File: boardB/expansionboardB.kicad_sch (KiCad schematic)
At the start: 45 parts, among them J1 USB_C_Receptacle, J3 HDMI_A, SW4 ESPPROG, U1 ESP32-S3-WROOM-1, U2 GPIO_U2, U4 GPIO_U4, U5 SII1136CTU, U7 MAX20022ATIA+T, t1V2 1V2_TEST, t3V3 3V3_TEST

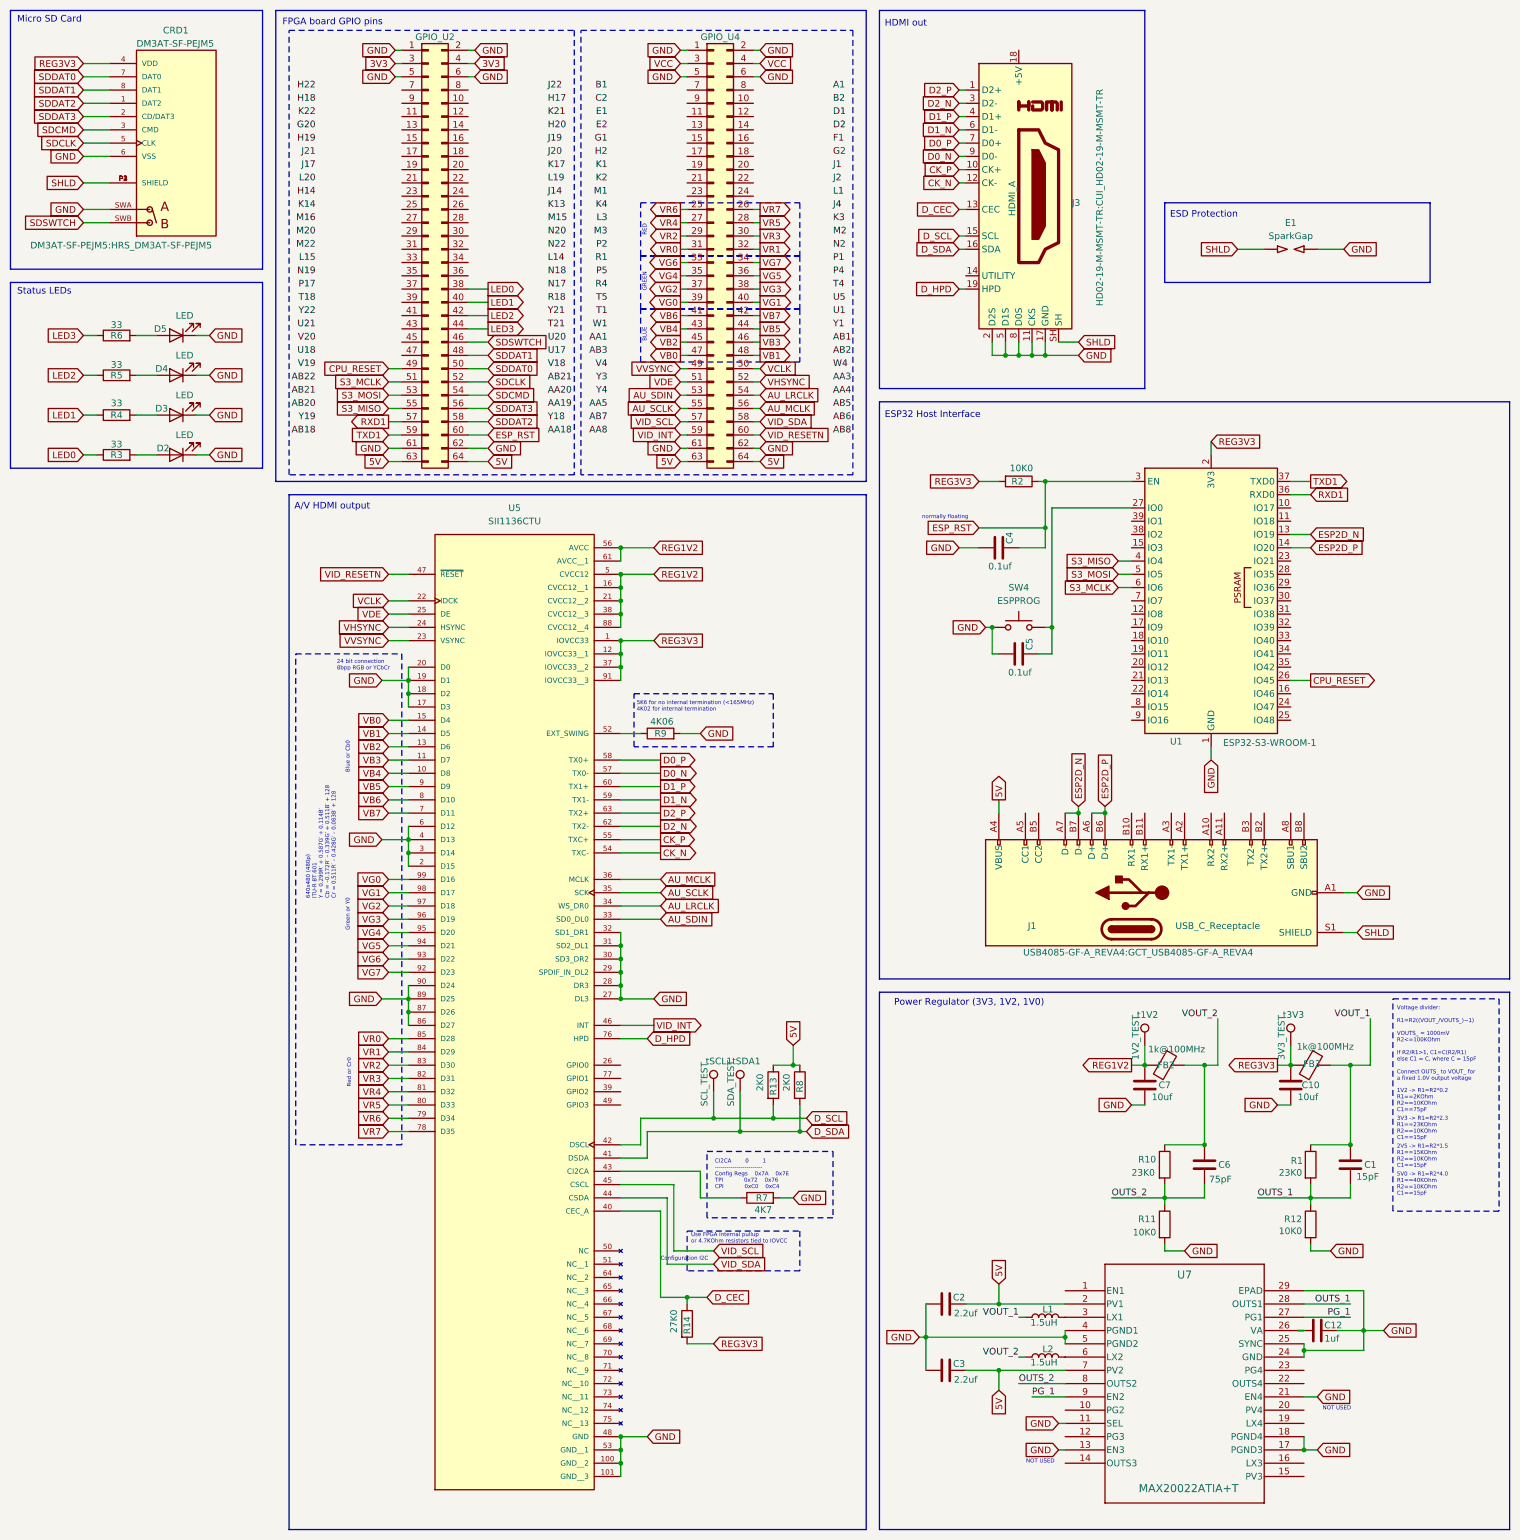
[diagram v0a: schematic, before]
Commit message: New board updates
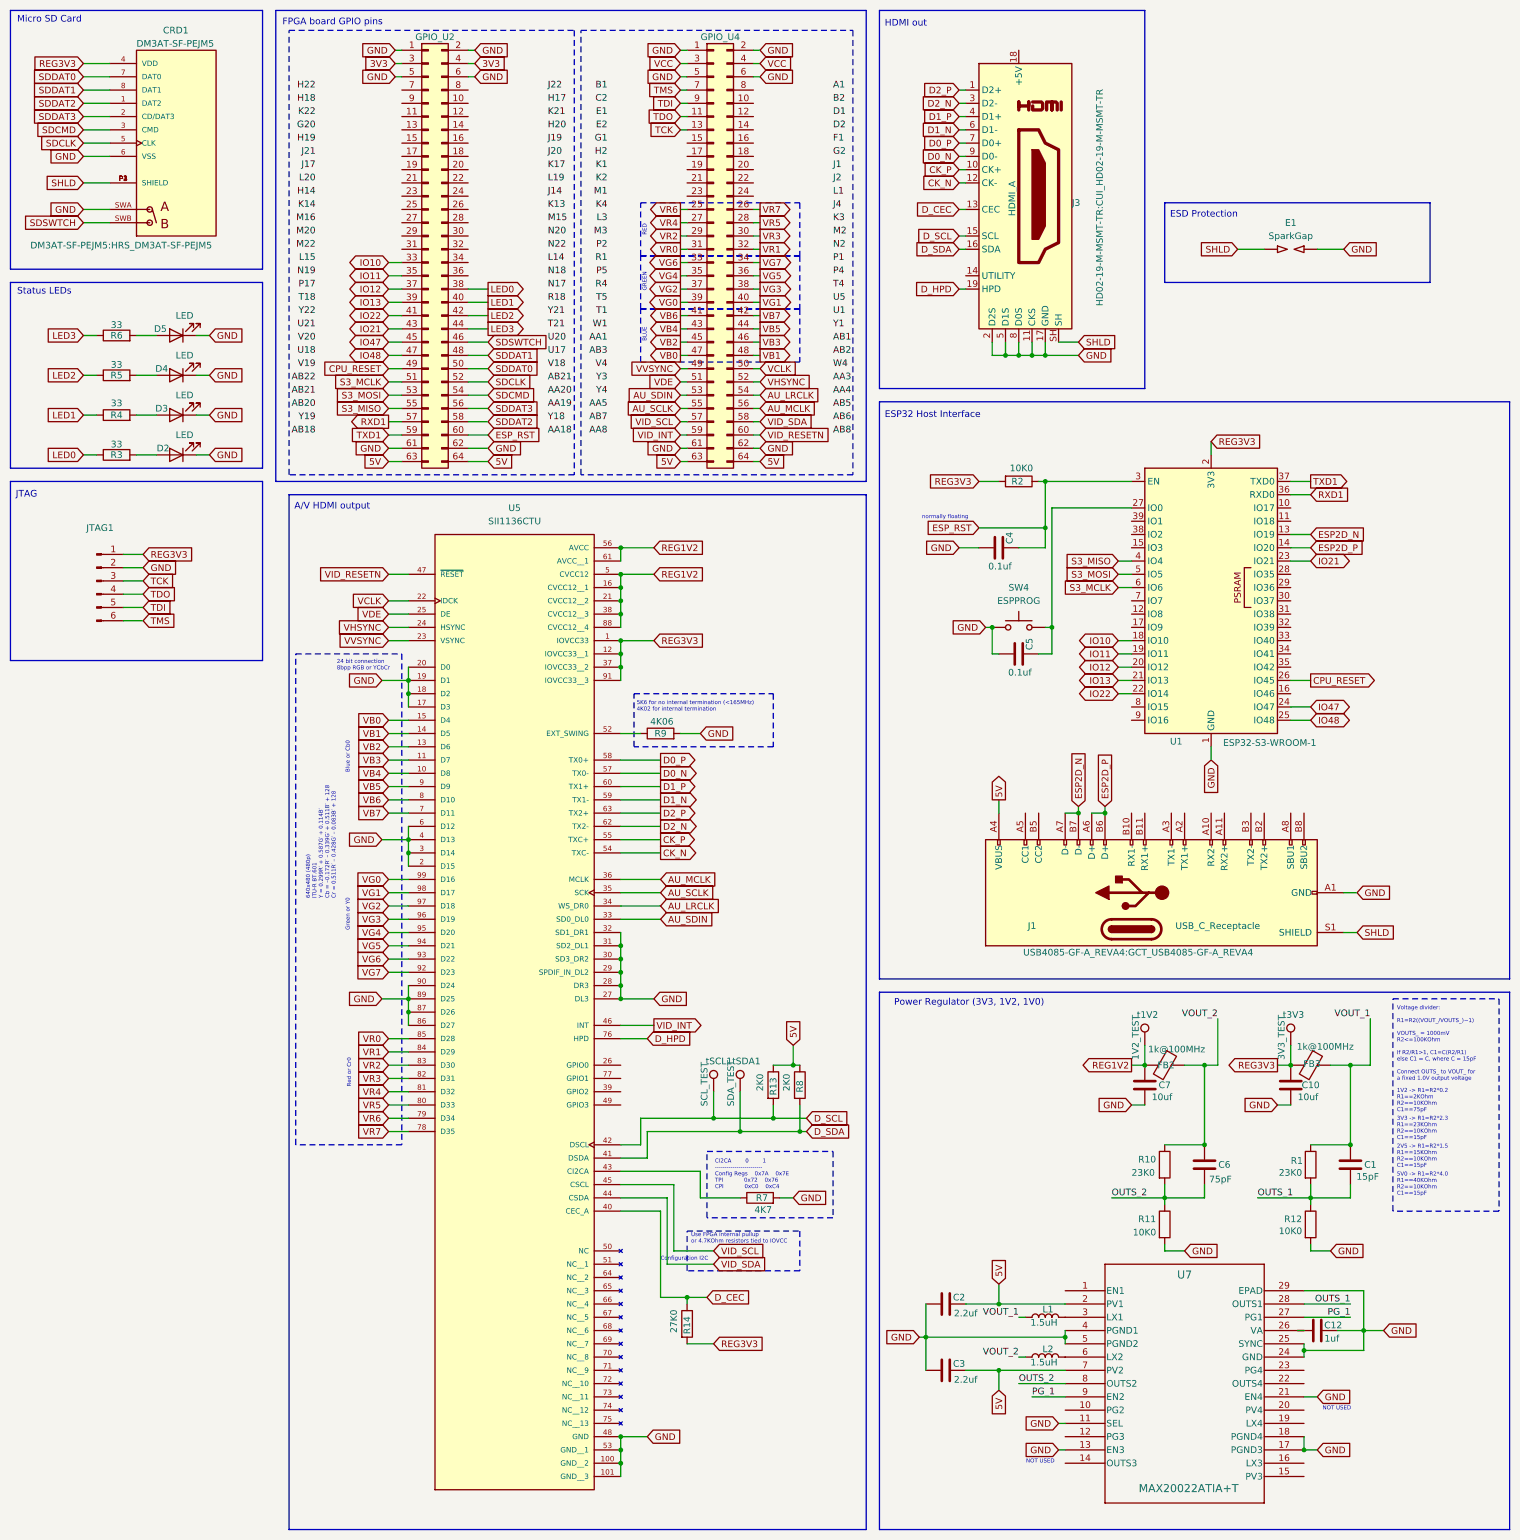
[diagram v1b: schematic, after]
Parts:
- added JTAG1: Conn_01x06_Pin, Connector_PinHeader_2.54mm:PinHeader_1x06_P2.54mm_Vertical, symbol Connector:Conn_01x06_Pin
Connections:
- net GND: now also JTAG1.2 (Pin_2)
- net REG3V3: now also JTAG1.1 (Pin_1)
- net IO10: now reaches U2.33 (Pin_33)
- net IO10: now also U1.18 (IO10)
- net IO11: now reaches U2.35 (Pin_35)
- net IO11: now also U1.19 (IO11)
- net IO12: now reaches U2.37 (Pin_37)
- net IO12: now also U1.20 (IO12)
- net IO13: now reaches U2.39 (Pin_39)
- net IO13: now also U1.21 (IO13)
- net IO22: now reaches U2.41 (Pin_41)
- net IO22: now also U1.22 (IO14)
- net IO21: now reaches U2.43 (Pin_43)
- net IO21: now also U1.23 (IO21)
- net IO47: now reaches U2.45 (Pin_45)
- net IO47: now also U1.24 (IO47)
- net IO48: now reaches U2.47 (Pin_47)
- net IO48: now also U1.25 (IO48)
- net TDO: now reaches U4.11 (Pin_11)
- net TDO: now also JTAG1.4 (Pin_4)
- net TCK: now reaches U4.13 (Pin_13)
- net TCK: now also JTAG1.3 (Pin_3)
- net TMS: now reaches U4.7 (Pin_7)
- net TMS: now also JTAG1.6 (Pin_6)
- net TDI: now reaches U4.9 (Pin_9)
- net TDI: now also JTAG1.5 (Pin_5)
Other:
- note added: "JTAG"
